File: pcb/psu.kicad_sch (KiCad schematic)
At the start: 7 parts, among them U1 LM78L05_SO8

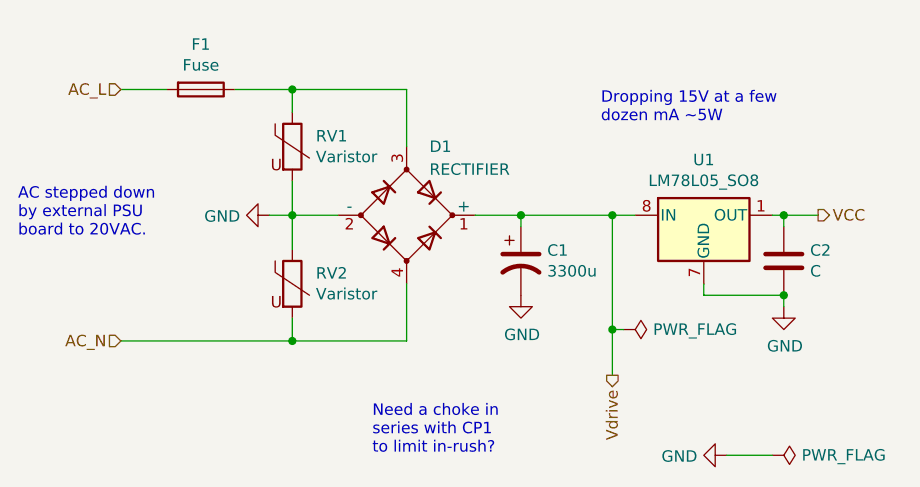
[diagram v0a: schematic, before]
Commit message: Tweak PSU
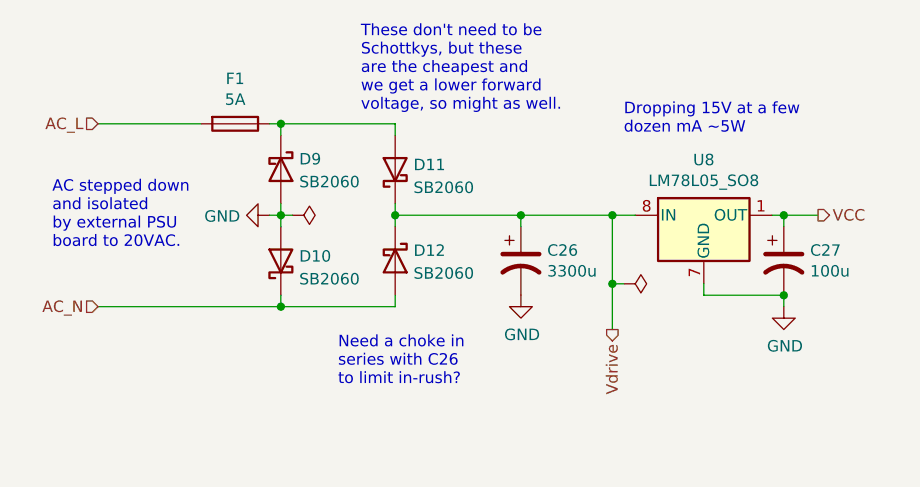
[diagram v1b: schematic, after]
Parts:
- removed C2: C, symbol Device:C
- removed D1: RECTIFIER, symbol Device:D_Bridge_+-AA
- removed RV1, RV2: Varistor, symbol Device:Varistor
- added C27: 100u, symbol Device:C_Polarized_US
- added D10, D11, D12, D9: SB2060, symbol Device:D_Schottky
- F1: value Fuse -> 5A
- renumbered C1 to C26, U1 to U8
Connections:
- net AC_N: now also D10.1 (K), D12.2 (A)
- net GND: now also C27.2, D10.2 (A), D9.2 (A)
- net VCC: now also C27.1
- net Vdrive: now also D11.1 (K), D12.1 (K)
- net at F1.1: now also D11.2 (A), D9.1 (K)
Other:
- note added: "AC stepped down and isolated by external PSU board to 20VAC."
- note added: "Need a choke in series with C26 to limit in-rush?"
- note added: "These don't need to be Schottkys, but these are the cheapest and we get a lower forward voltage, so might as well."
- note removed: "AC stepped down by external PSU board to 20VAC."
- note removed: "Need a choke in series with CP1 to limit in-rush?"
- title: (none) -> Power Supply
- moved on the sheet: F1
